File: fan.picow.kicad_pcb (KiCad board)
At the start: 2 copper layers, 60.3 x 65.7 mm, 53 parts, among them J10 5v Input, J11 12v Input, J12 Temp DHT22, J2 Fan1 Conn, J3 Fan2 Conn, J4 Fan4 Conn, J5 Fan3 Conn, J6 Buzz Conn, J7 OLED, J8 Relay Ctrl, J9 Relay Out, U1 PicoW

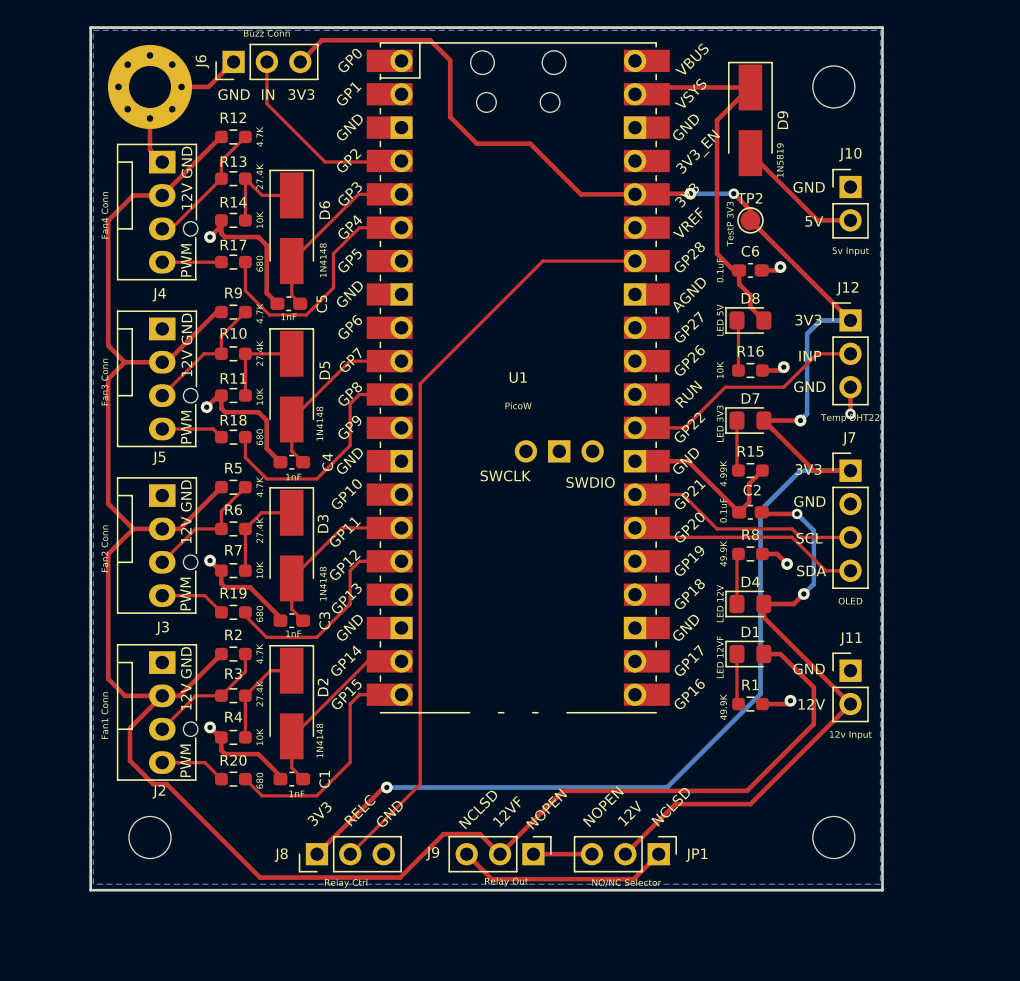
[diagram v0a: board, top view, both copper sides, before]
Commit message: pop stashed changes
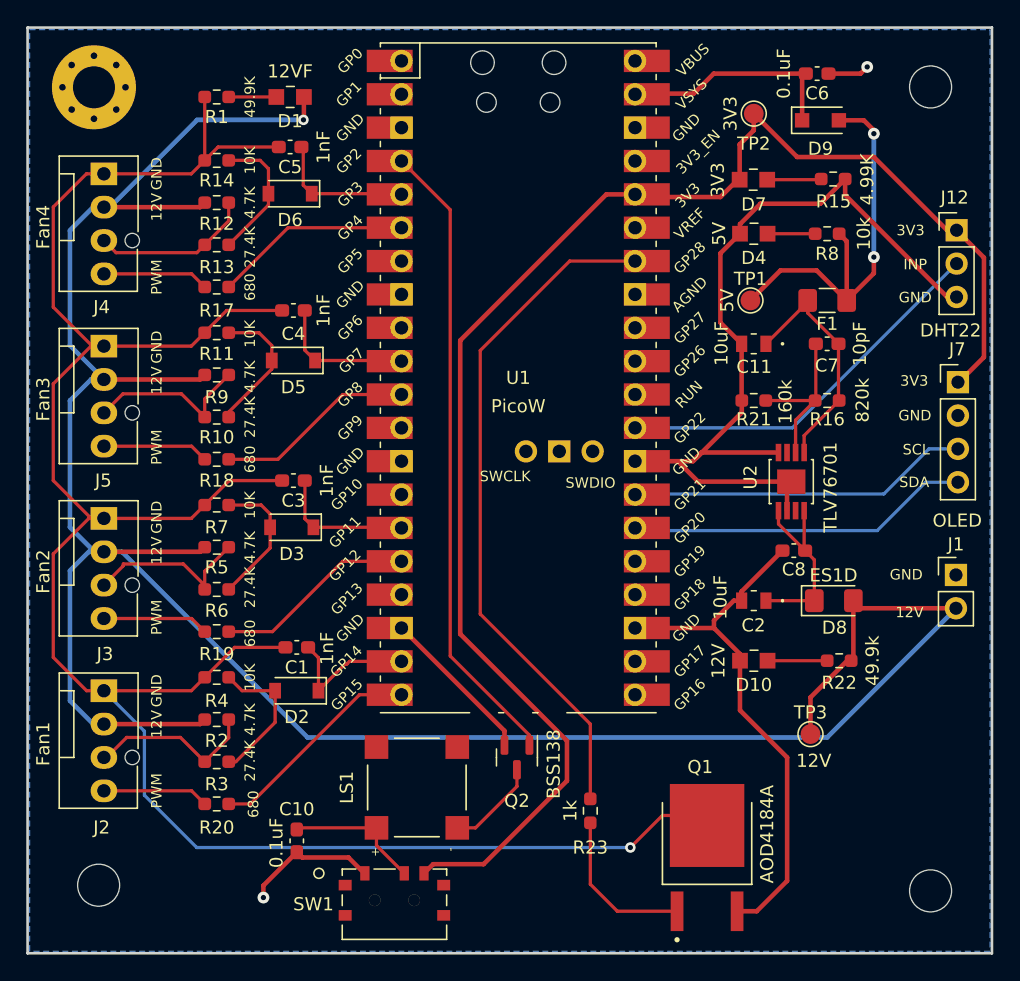
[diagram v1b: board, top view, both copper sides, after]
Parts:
- removed J10: 5v Input, Connector_PinHeader_2.54mm:PinHeader_1x02_P2.54mm_Vertical
- removed J11: 12v Input, Connector_PinHeader_2.54mm:PinHeader_1x02_P2.54mm_Vertical
- removed J6: Buzz Conn, Connector_PinHeader_2.54mm:PinHeader_1x03_P2.54mm_Vertical
- removed J8: Relay Ctrl, Connector_PinHeader_2.54mm:PinHeader_1x03_P2.54mm_Vertical
- removed J9: Relay Out, Connector_PinHeader_2.54mm:PinHeader_1x03_P2.54mm_Vertical
- removed JP1: NO/NC Selector, Connector_PinHeader_2.54mm:PinHeader_1x03_P2.54mm_Vertical
- added C10: 0.1uF, Capacitor_SMD:C_0603_1608Metric_Pad1.08x0.95mm_HandSolder, F.Cu at (130.6, 103.1)
- added C11: 10uF, footprints descargados:CL21A106KOQNNNE, F.Cu at (165.4, 65.3)
- added C7: 10pF, Capacitor_SMD:C_0603_1608Metric_Pad1.08x0.95mm_HandSolder, F.Cu at (170.9, 65.3)
- added C8: 1uF, Capacitor_SMD:C_0603_1608Metric_Pad1.08x0.95mm_HandSolder, F.Cu at (168.4, 81.0)
- added D10: 12V, digikey-footprints:0805, F.Cu at (165.4, 89.4)
- added F1: Polyfuse 0.5A, Fuse:Fuse_1206_3216Metric_Pad1.42x1.75mm_HandSolder, F.Cu at (170.9, 62.0)
- added J1: 12v Input, Connector_PinHeader_2.54mm:PinHeader_1x02_P2.54mm_Vertical, F.Cu at (180.7, 82.9)
- added LS1: CMT-7525-80-SMT-TR, footprints descargados:XDCR_CMT-7525-80-SMT-TR, F.Cu at (139.7, 99.1)
- added Q1: AOD4184A, footprints descargados:DPAK228P994X240-4N, F.Cu at (161.8, 104.4)
- added Q2: BSS138, Package_TO_SOT_SMD:SOT-23, F.Cu at (147.3, 96.8)
- added R21: 160k, Resistor_SMD:R_0603_1608Metric_Pad0.98x0.95mm_HandSolder, F.Cu at (165.4, 69.6)
- added R22: 49.9k, Resistor_SMD:R_0603_1608Metric_Pad0.98x0.95mm_HandSolder, F.Cu at (171.9, 89.4)
- added R23: 1k, Resistor_SMD:R_0603_1608Metric_Pad0.98x0.95mm_HandSolder, F.Cu at (152.9, 100.8)
- added SW1: EG1257, footprints descargados:EG1257, F.Cu at (138.0, 108.0)
- added TP1: 5V, TestPoint:TestPoint_Pad_D1.5mm, F.Cu at (165.1, 62.0)
- added TP3: 12V, TestPoint:TestPoint_Pad_D1.5mm, F.Cu at (169.7, 95.0)
- added U2: TLV76701, footprints descargados:TLV76701DGNR, F.Cu at (168.2, 75.8)
- C2: value 0.1uF -> 10uF; footprint Capacitor_SMD:C_0603_1608Metric_Pad1.08x0.95mm_HandSolder -> footprints descargados:CL21A106KOQNNNE
- D1: value LED 12VF -> 12VF; footprint LED_SMD:LED_0805_2012Metric_Pad1.15x1.40mm_HandSolder -> digikey-footprints:0805
- D2, D3, D5, D6: footprint Diode_SMD:D_SMA_Handsoldering -> Diode_SMD:D_SOD-123
- D4: value LED 12V -> 5V; footprint LED_SMD:LED_0805_2012Metric_Pad1.15x1.40mm_HandSolder -> digikey-footprints:0805
- D7: value LED 3V3 -> 3V3; footprint LED_SMD:LED_0805_2012Metric_Pad1.15x1.40mm_HandSolder -> digikey-footprints:0805
- D8: value LED 5V -> ES1D; footprint LED_SMD:LED_0805_2012Metric_Pad1.15x1.40mm_HandSolder -> Diode_SMD:D_1206_3216Metric_Pad1.42x1.75mm_HandSolder
- D9: value 1N5819 -> CDBW140-G; footprint Diode_SMD:D_SMA_Handsoldering -> Diode_SMD:D_SOD-123F
- J12: value Temp DHT22 -> DHT22
- J2: value Fan1 Conn -> Fan1
- J3: value Fan2 Conn -> Fan2
- J4: value Fan4 Conn -> Fan4
- J5: value Fan3 Conn -> Fan3
- R16: value 10K -> 820k
- R8: value 49.9K -> 10k
- TP2: value TestP 3V3 -> 3V3
- moved R1 61.6 mm to (124.5, 46.5), turned to 180 degrees
- moved D1 55.0 mm to (130.0, 46.5), turned to 180 degrees
- moved D4 28.2 mm to (165.4, 56.9), turned to 180 degrees
- moved R8 25.1 mm to (170.9, 56.9), turned to 180 degrees
- moved R15 23.1 mm to (171.4, 52.7)
- moved D8 22.3 mm to (171.4, 84.8)
- moved D7 18.3 mm to (165.3, 52.8)
- moved C6 15.8 mm to (170.2, 44.7)
- moved C5 11.9 mm to (130.0, 50.3)
- moved C4 11.6 mm to (130.3, 62.7)
- moved C3 10.7 mm to (130.3, 75.7)
- moved J12 10.6 mm to (180.8, 56.6)
- moved J7 10.6 mm to (180.9, 68.2)
- moved C1 10.0 mm to (130.6, 88.4)
- moved H3 8.41 mm to (178.8, 106.9)
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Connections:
- C1 pad 2: GND -> /GNDFAN
- C2 pad 1: /12V -> Net-(C2-Pad1)
- C3 pad 2: GND -> /GNDFAN
- C4 pad 2: GND -> /GNDFAN
- C5 pad 2: GND -> /GNDFAN
- D1 pad 1: Net-(D1-Pad1) -> /12V
- D1 pad 2: /12VFAN -> Net-(D1-Pad2)
- D2 pad 1: Net-(D2-Pad1) -> /TACHM1
- D2 pad 2: /TACHM1 -> Net-(D2-Pad2)
- D3 pad 1: Net-(D3-Pad1) -> /TACHM2
- D3 pad 2: /TACHM2 -> Net-(D3-Pad2)
- D4 pad 2: /12V -> GND
- D5 pad 1: Net-(D5-Pad1) -> /TACHM3
- D5 pad 2: /TACHM3 -> Net-(D5-Pad2)
- D6 pad 1: Net-(D6-Pad1) -> /TACHM4
- D6 pad 2: /TACHM4 -> Net-(D6-Pad2)
- D7 pad 1: Net-(D7-Pad1) -> /3V3
- D7 pad 2: /3V3 -> Net-(D7-Pad2)
- D8 pad 1: Net-(D8-Pad1) -> Net-(C2-Pad1)
- D8 pad 2: /VSYS -> /12V
- J2 pad 1: GND -> /GNDFAN
- J2 pad 2: /12VFAN -> /12V
- J3 pad 1: GND -> /GNDFAN
- J3 pad 2: /12VFAN -> /12V
- J4 pad 1: GND -> /GNDFAN
- J4 pad 2: /12VFAN -> /12V
- J5 pad 1: GND -> /GNDFAN
- J5 pad 2: /12VFAN -> /12V
- R1 pad 1: Net-(D1-Pad1) -> Net-(D1-Pad2)
- R1 pad 2: GND -> /GNDFAN
- R10 pad 2: Net-(D5-Pad1) -> Net-(D5-Pad2)
- R11 pad 1: Net-(D5-Pad1) -> Net-(D5-Pad2)
- R11 pad 2: GND -> /GNDFAN
- R12 pad 1: /12VFAN -> /12V
- R13 pad 2: Net-(D6-Pad1) -> Net-(D6-Pad2)
- R14 pad 1: Net-(D6-Pad1) -> Net-(D6-Pad2)
- R14 pad 2: GND -> /GNDFAN
- R15 pad 1: Net-(D7-Pad1) -> Net-(D7-Pad2)
- R16 pad 1: Net-(D8-Pad1) -> Net-(C11-Pad1)
- R16 pad 2: GND -> Net-(C7-Pad2)
- R2 pad 1: /12VFAN -> /12V
- R3 pad 2: Net-(D2-Pad1) -> Net-(D2-Pad2)
- R4 pad 1: Net-(D2-Pad1) -> Net-(D2-Pad2)
- R4 pad 2: GND -> /GNDFAN
- R5 pad 1: /12VFAN -> /12V
- R6 pad 2: Net-(D3-Pad1) -> Net-(D3-Pad2)
- R7 pad 1: Net-(D3-Pad1) -> Net-(D3-Pad2)
- R7 pad 2: GND -> /GNDFAN
- R8 pad 1: Net-(D4-Pad1) -> /5V
- R8 pad 2: GND -> Net-(D4-Pad1)
- R9 pad 1: /12VFAN -> /12V
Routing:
- net /GNDFAN: track 0.00 -> 171.3 mm, vias 0 -> 1
- net /12VFAN: track 151.7 -> 0.00 mm
- net /12V: track 45.3 -> 194.0 mm, vias 2 -> 1
- net GND: track 68.5 -> 132.1 mm, vias 9 -> 2
- net /BUZZ: track 15.3 -> 48.5 mm
- net /3V3: track 136.8 -> 115.1 mm, vias 4 -> 0
- net /5V: track 9.74 -> 31.3 mm, vias 0 -> 2
- net Net-(C11-Pad1): track 0.00 -> 18.3 mm
- net /conectores/NCLOSED: track 16.2 -> 0.00 mm
- net Net-(C2-Pad1): track 0.00 -> 14.7 mm
- net Net-(C7-Pad2): track 0.00 -> 12.7 mm
- net /VSYS: track 29.5 -> 17.3 mm
- net Net-(Q1-Pad1): track 0.00 -> 12.1 mm
- net Net-(D2-Pad2): track 0.00 -> 11.1 mm
- net /TEMPHUM: track 18.7 -> 29.7 mm
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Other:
- board size 60.3 x 65.7 mm -> 73.4 x 70.5 mm
- board text added: "0.2000 mm / 0.0000 mm"
- board text added: "0.3000 mm"
- board text added: "1.6000 mm"
- board text added: "2"
- board text added: "60.2996 mm x 65.6844 mm"
- board text added: "BOARD CHARACTERISTICS"
- board text added: "Board Thickness:"
- board text added: "Board overall dimensions:"
- board text added: "Castellated pads:"
- board text added: "Copper Finish:"
- board text added: "Copper Layer Count:"
- board text added: "Edge card connectors:"
- board text added: "Falta: - Graficos detras - Version de la placa - Iniciales - Tamaño de la placa (para caja standard) y posicion agujeros - Redondear los bordes (cambiar rectangulo por lineas) - Tamaños de los componentes"
- board text added: "Fan Controller v0.1 Based on RaspberryPi PicoW MCU"
- board text added: "Impedance Control:"
- board text added: "Min hole diameter:"
- board text added: "Min track/spacing:"
- board text added: "No"
- board text added: "None"
- board text added: "Plated Board Edge:"
- board text added: "by Jaime Botella jimbotel@gmail.com 2022/11"
- board text removed: "12VF"
- board text removed: "5V"
- board text removed: "Falta: - Graficos detras - Version de la placa - Iniciales - Validar valores Rs de LEDs - Tamaños de los componentes"
- board text removed: "IN"
- board text removed: "NCLSD"
- board text removed: "NOPEN"
- board text removed: "RELC"
